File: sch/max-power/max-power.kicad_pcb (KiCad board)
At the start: 2 copper layers, 150 x 180 mm, 47 parts, among them P1 CONN_01X04, P10 CONN_01X09, P12 CONN_02X06, P13 CONN_02X04, P2 CONN_01X04, P3 ATX-PWR-24P, P4 CONN_02X05, P5 CONN_01X09, P6 CONN_01X02, P7 CONN_01X02, P8 CONN_01X09, P9 CONN_01X09, Q1 2N7002, SW1 SW_PUSH

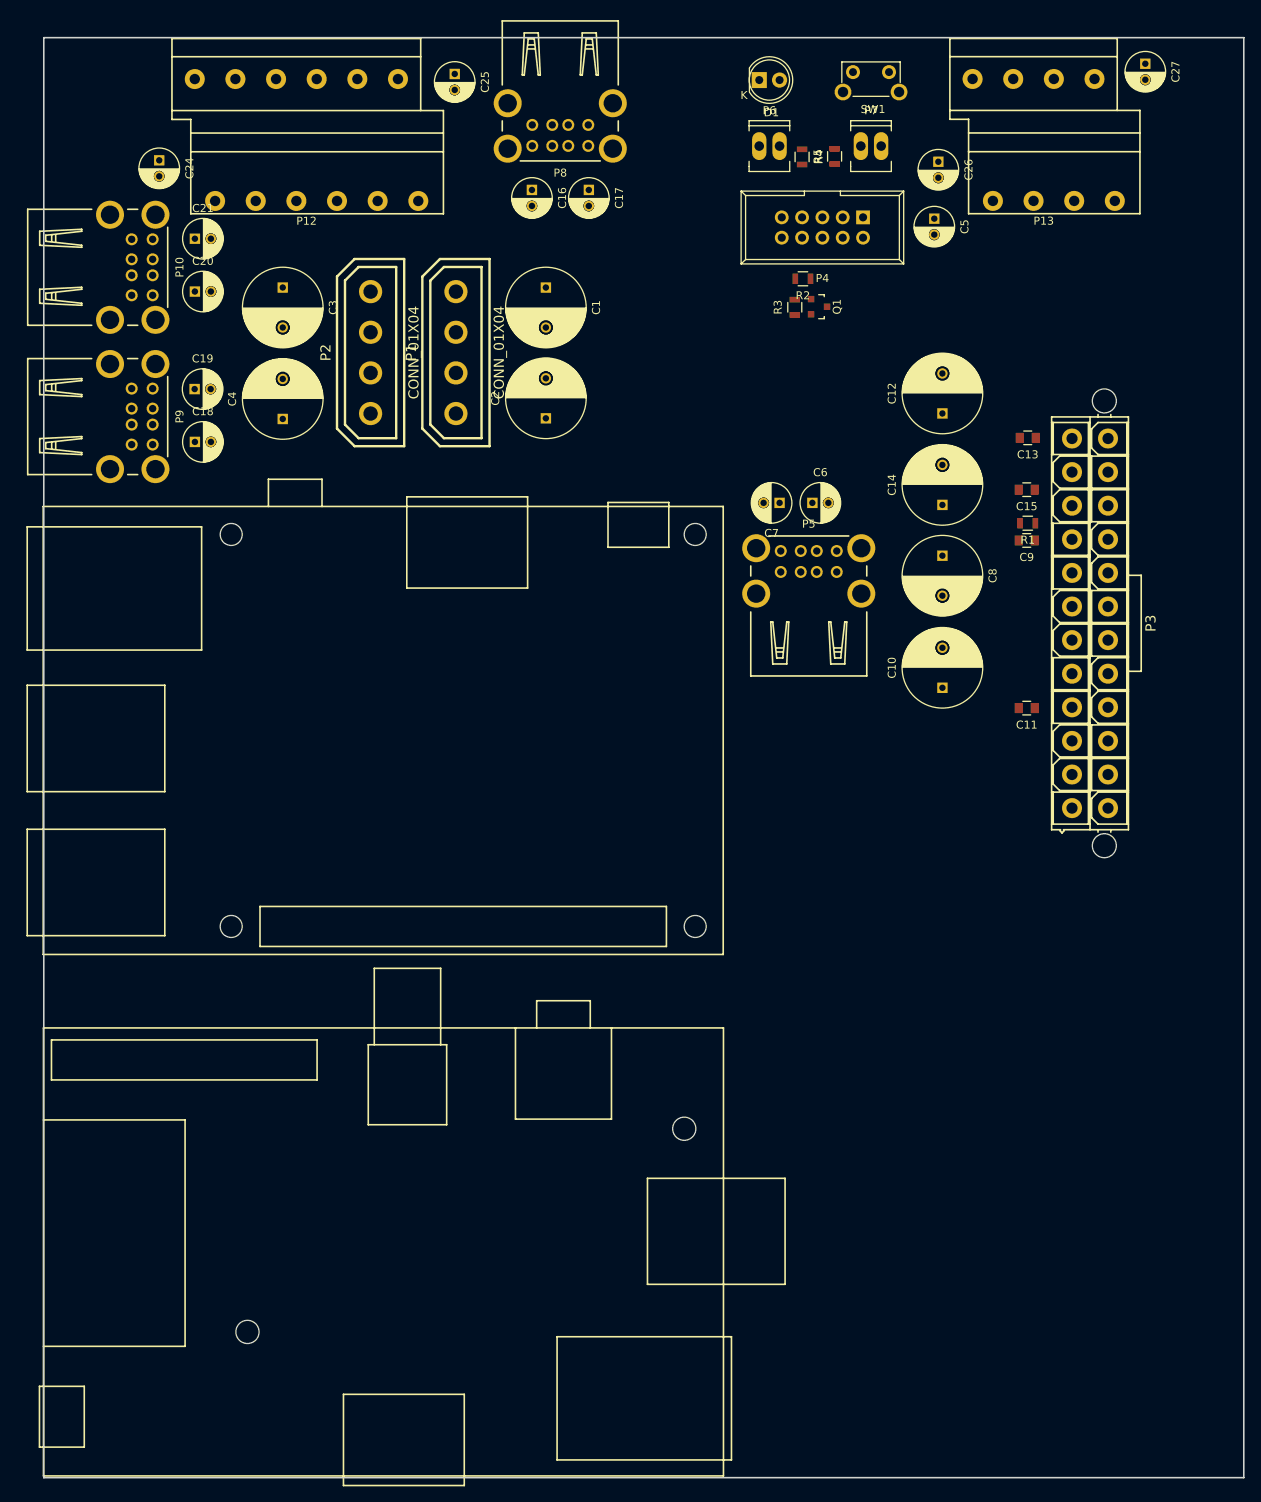
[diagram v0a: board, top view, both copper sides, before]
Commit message: Routed PCB.
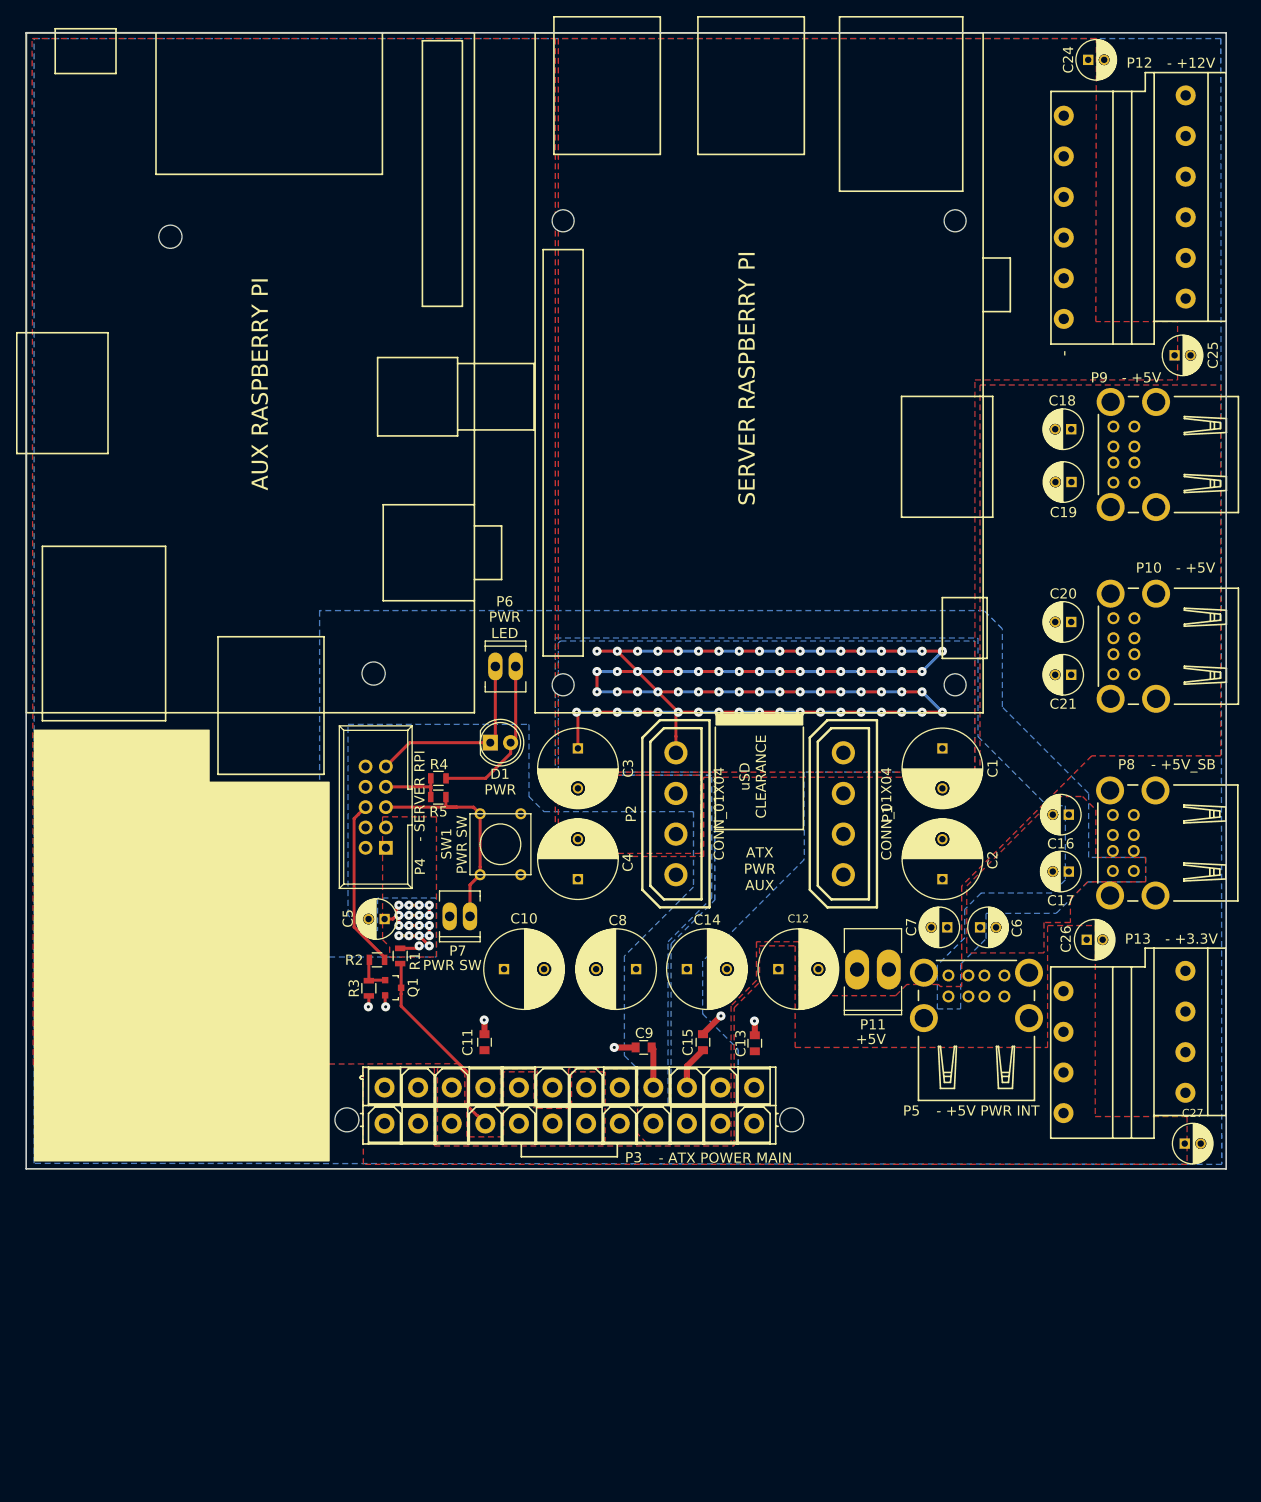
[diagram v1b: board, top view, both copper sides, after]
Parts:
- added P11: CONN_01X02, Sockets_MOLEX_KK-System:Socket_MOLEX-KK-RM3-96mm_Lock_2pin_straight, F.Cu at (123.4, 132.5)
- SW1: footprint Buttons_Switches_THT:SW_Tactile_SPST_Angled -> Buttons_Switches_THT:SW_PUSH_SMALL
- moved C27 135.1 mm to (162.4, 154.3), turned to 0 degrees
- moved P10 134.0 mm to (156.1, 92.1), turned to 90 degrees
- moved P9 125.4 mm to (156.1, 68.1), turned to 90 degrees
- moved C21 122.4 mm to (148.2, 95.7), turned to 180 degrees
- moved C20 117.1 mm to (148.2, 89.1), turned to 180 degrees
- moved C24 116.8 mm to (150.3, 18.8), turned to 0 degrees
- moved P8 114.9 mm to (156.0, 116.7), turned to 90 degrees
- moved P13 113.2 mm to (154.8, 141.6), turned to 90 degrees
- moved C5 111.3 mm to (62.4, 126.2), turned to 180 degrees
- moved REF** 111.2 mm to (45.6, 57.9), turned to 270 degrees
- moved C19 110.2 mm to (148.2, 71.6), turned to 180 degrees
- moved C18 109.6 mm to (148.2, 65.0), turned to 180 degrees
- moved P7 109.1 mm to (71.8, 125.9), turned to 180 degrees
- moved SW1 106.1 mm to (76.8, 116.8), turned to 90 degrees
- moved C17 104.2 mm to (147.9, 120.3), turned to 180 degrees
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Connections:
- P12 pad 1: +12V -> GND
- P12 pad 10: GND -> +12V
- P12 pad 11: +12V -> GND
- P12 pad 12: GND -> +12V
- P12 pad 2: GND -> +12V
- P12 pad 3: +12V -> GND
- P12 pad 4: GND -> +12V
- P12 pad 5: +12V -> GND
- P12 pad 6: GND -> +12V
- P12 pad 7: +12V -> GND
- P12 pad 8: GND -> +12V
- P12 pad 9: +12V -> GND
- P13 pad 1: +3V3 -> GND
- P13 pad 2: GND -> +3V3
- P13 pad 3: +3V3 -> GND
- P13 pad 4: GND -> +3V3
- P13 pad 5: +3V3 -> GND
- P13 pad 6: GND -> +3V3
- P13 pad 7: +3V3 -> GND
- P13 pad 8: GND -> +3V3
- P4 pad 5: /PS_ON -> /PWR_SW
- P4 pad 6: /PWR_SW -> /PS_ON
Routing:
- net +12V: track 0.00 -> 205.7 mm, vias 0 -> 71
- net +5VP: track 0.00 -> 35.3 mm, vias 0 -> 18
- net /PWR_SW: track 0.00 -> 28.0 mm
- net Net-(P3-Pad16): track 0.00 -> 24.4 mm
- net Net-(D1-Pad1): track 0.00 -> 24.1 mm
- net /PS_ON: track 0.00 -> 21.3 mm
- net Net-(D1-Pad2): track 0.00 -> 20.5 mm
- net GND: track 0.00 -> 12.3 mm, vias 0 -> 6
- net /3.3VPI: track 0.00 -> 7.96 mm
- net Net-(Q1-Pad1): track 0.00 -> 4.69 mm
- added copper zone on B.Cu, net +12V
- added copper zone on F.Cu, net +12V
- added copper zone on F.Cu, net +3V3
- added copper zone on F.Cu, net +5V
- added copper zone on B.Cu, net +5VP
- added copper zone on F.Cu, net +5VP
- added copper zone on B.Cu, net GND
- added copper zone on F.Cu, net GND
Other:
- board size 150 x 180 mm -> 150 x 142 mm
- net class Default: clearance 0.2 -> 0.381; trace_width 0.25 -> 0.381; via_dia 0.8 -> 1.143; via_drill 0.4 -> 0.381
- rule trace_clearance: 0.2 -> 0.381
- rule trace_min: 0.2 -> 0.381
- rule via_min_drill: 0.3 -> 0.381
- rule via_min_size: 0.4 -> 1.143
- board text added: "+5V"
- board text added: "-"
- board text added: "- +12V"
- board text added: "- +3.3V"
- board text added: "- +5V"
- board text added: "- +5V PWR INT"
- board text added: "- +5V_SB"
- board text added: "- ATX POWER MAIN"
- board text added: "- SERVER RPI"
- board text added: "ATX PSU measurements: 150x142x86 mm"
- board text added: "ATX PWR AUX"
- board text added: "AUX RASPBERRY PI"
- board text added: "PWR"
- board text added: "PWR LED"
- board text added: "PWR SW"
- board text added: "SERVER RASPBERRY PI"
- board text added: "uSD CLEARANCE"
- board text removed: "ATX PSU measurements: 180x150x86 mm"
